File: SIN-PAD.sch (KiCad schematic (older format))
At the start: 1 part

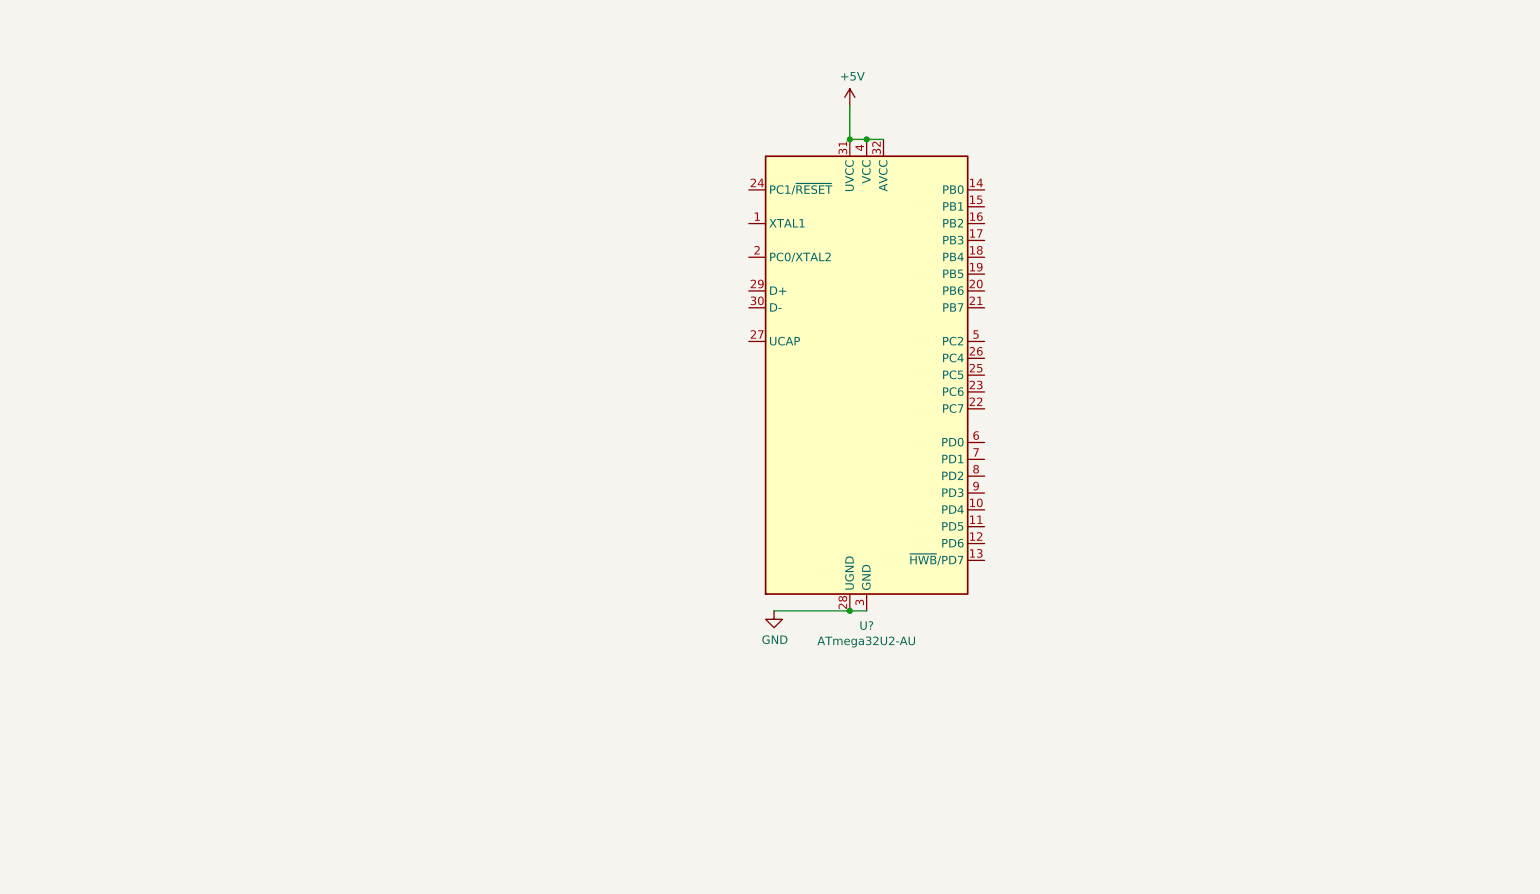
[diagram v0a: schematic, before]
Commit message: Big brain commit 23:36
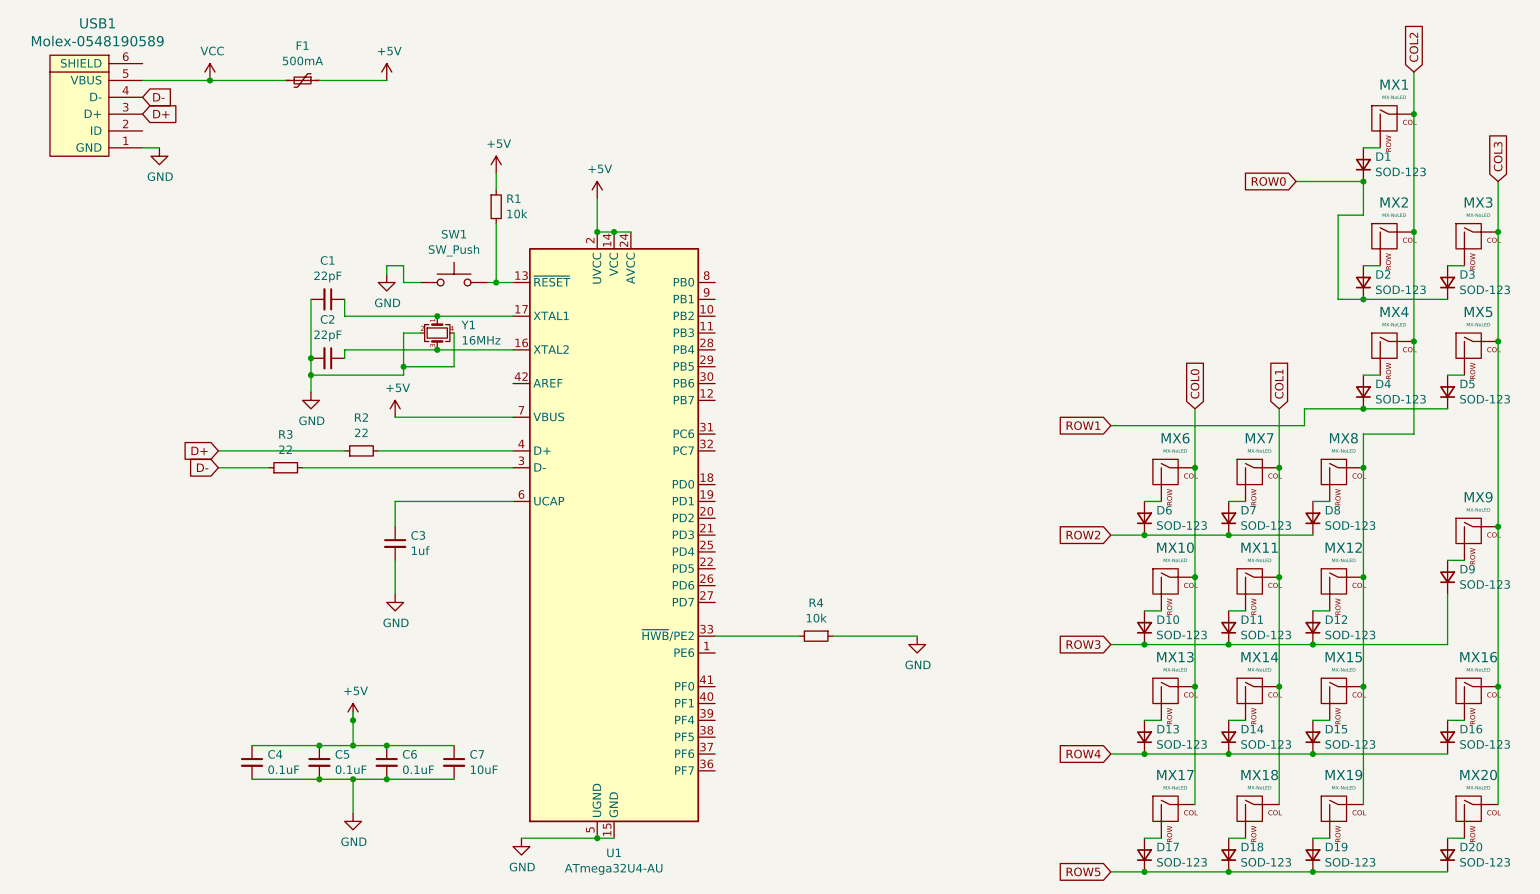
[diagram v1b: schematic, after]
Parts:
- removed U?: ATmega32U2-AU, Package_QFP:TQFP-32_7x7mm_P0.8mm, symbol MCU_Microchip_ATmega:ATmega32U2-AU
- added C1, C2: 22pF, Capacitor_SMD:C_0805_2012Metric, symbol Device:C_Small
- added C3: 1uf, Capacitor_SMD:C_0805_2012Metric, symbol Device:C_Small
- added C4, C5, C6: 0.1uF, Capacitor_SMD:C_0805_2012Metric, symbol Device:C_Small
- added C7: 10uF, Capacitor_SMD:C_0805_2012Metric, symbol Device:C_Small
- added D1, D10, D11, D12, D13, D14, D15, D16, D17, D18, D19, D2, D20, D3, D4, D5, D6, D7, D8, D9: SOD-123, Diode_SMD:D_SOD-123, symbol Device:D_Small
- added F1: 500mA, Fuse:Fuse_1206_3216Metric, symbol Device:Polyfuse_Small
- added MX1, MX10, MX11, MX12, MX13, MX14, MX15, MX16, MX17, MX18, MX19, MX2, MX20, MX3, MX4, MX5, MX6, MX7, MX8: MX-NoLED, MX_Only:MXOnly-1U-NoLED, symbol MX_Alps_Hybrid:MX-NoLED
- added MX9: MX-NoLED, MX_Only:MXOnly-2U-NoLED, symbol MX_Alps_Hybrid:MX-NoLED
- added R1, R4: 10k, Resistor_SMD:R_0805_2012Metric, symbol Device:R_Small
- added R2, R3: 22, Resistor_SMD:R_0805_2012Metric, symbol Device:R_Small
- added SW1: SW_Push, random-keyboard-parts:SKQG-1155865, symbol Switch:SW_Push
- added U1: ATmega32U4-AU, Package_QFP:TQFP-44_10x10mm_P0.8mm, symbol MCU_Microchip_ATmega:ATmega32U4-AU
- added USB1: Molex-0548190589, random-keyboard-parts:Molex-0548190589, symbol random-keyboard-parts:Molex-0548190589
- added Y1: 16MHz, Crystal:Crystal_SMD_3225-4Pin_3.2x2.5mm, symbol Device:Crystal_GND24_Small
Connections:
- net +5V: now also C4.1, C5.1, C6.1, C7.1, F1.1, R1.1, U1.14 (VCC), U1.2 (UVCC), U1.24 (AVCC), U1.34 (VCC), U1.44 (AVCC), U1.7 (VBUS)
- net GND: now also C1.2, C2.2, C3.2, C4.2, C5.2, C6.2, C7.2, R4.1, SW1.1, U1.15 (GND), U1.23 (GND), U1.35 (GND), U1.43 (GND), U1.5 (UGND), USB1.1 (GND), Y1.2, Y1.4
- new net: R4.2, U1.33 (~HWB~/PE2)
- new net: R1.2, SW1.2, U1.13 (~RESET)
- new net: C2.1, U1.16 (XTAL2), Y1.3
- new net: C1.1, U1.17 (XTAL1), Y1.1
- new net: R3.2, U1.3 (D-)
- new net: R2.2, U1.4 (D+)
- new net: C3.1, U1.6 (UCAP)
- new net: D6.2 (A), MX6.2 (ROW)
- new net: D7.2 (A), MX7.2 (ROW)
- new net: D10.2 (A), MX10.2 (ROW)
- new net: D11.2 (A), MX11.2 (ROW)
- new net: D8.2 (A), MX8.2 (ROW)
- new net: D9.2 (A), MX9.2 (ROW)
- new net: D12.2 (A), MX12.2 (ROW)
- new net: D16.2 (A), MX16.2 (ROW)
- new net: D13.2 (A), MX13.2 (ROW)
- new net: D14.2 (A), MX14.2 (ROW)
- new net: D17.2 (A), MX17.2 (ROW)
- new net: D18.2 (A), MX18.2 (ROW)
- new net: D15.2 (A), MX15.2 (ROW)
- new net: D19.2 (A), MX19.2 (ROW)
- new net: D20.2 (A), MX20.2 (ROW)
- new net: D2.2 (A), MX2.2 (ROW)
- new net: D3.2 (A), MX3.2 (ROW)
- new net: D4.2 (A), MX4.2 (ROW)
- new net: D5.2 (A), MX5.2 (ROW)
- new net: D1.2 (A), MX1.2 (ROW)
- new net COL0: MX10.1 (COL), MX13.1 (COL), MX17.1 (COL), MX6.1 (COL)
- new net COL1: MX11.1 (COL), MX14.1 (COL), MX18.1 (COL), MX7.1 (COL)
- new net COL2: MX1.1 (COL), MX12.1 (COL), MX15.1 (COL), MX19.1 (COL), MX2.1 (COL), MX4.1 (COL), MX8.1 (COL)
- new net COL3: MX16.1 (COL), MX20.1 (COL), MX3.1 (COL), MX5.1 (COL), MX9.1 (COL)
- new net D+: R2.1, USB1.3 (D+)
- new net D-: R3.1, USB1.4 (D-)
- new net ROW0: D1.1 (K), D2.1 (K), D3.1 (K)
- new net ROW1: D4.1 (K), D5.1 (K)
- new net ROW2: D6.1 (K), D7.1 (K), D8.1 (K)
- new net ROW3: D10.1 (K), D11.1 (K), D12.1 (K), D9.1 (K)
- new net ROW4: D13.1 (K), D14.1 (K), D15.1 (K), D16.1 (K)
- new net ROW5: D17.1 (K), D18.1 (K), D19.1 (K), D20.1 (K)
- new net VCC: F1.2, USB1.5 (VBUS)
